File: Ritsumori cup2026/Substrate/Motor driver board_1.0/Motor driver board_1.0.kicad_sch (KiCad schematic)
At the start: 49 parts, among them J1 main, U1 DRV8412, U2 DRV8412

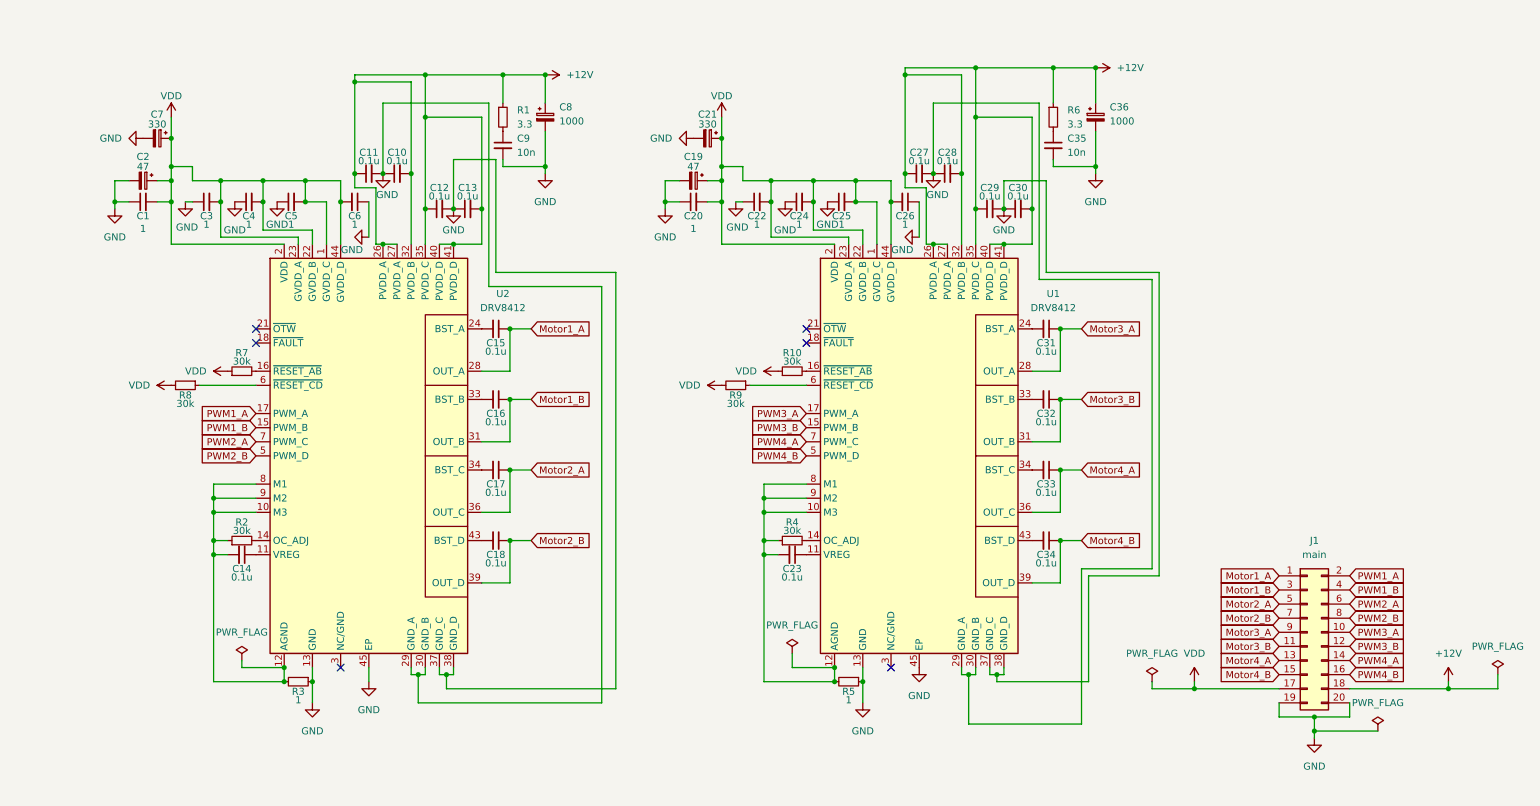
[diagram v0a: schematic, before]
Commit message: Auto Backup: 2026/03/24 15:00:23.58
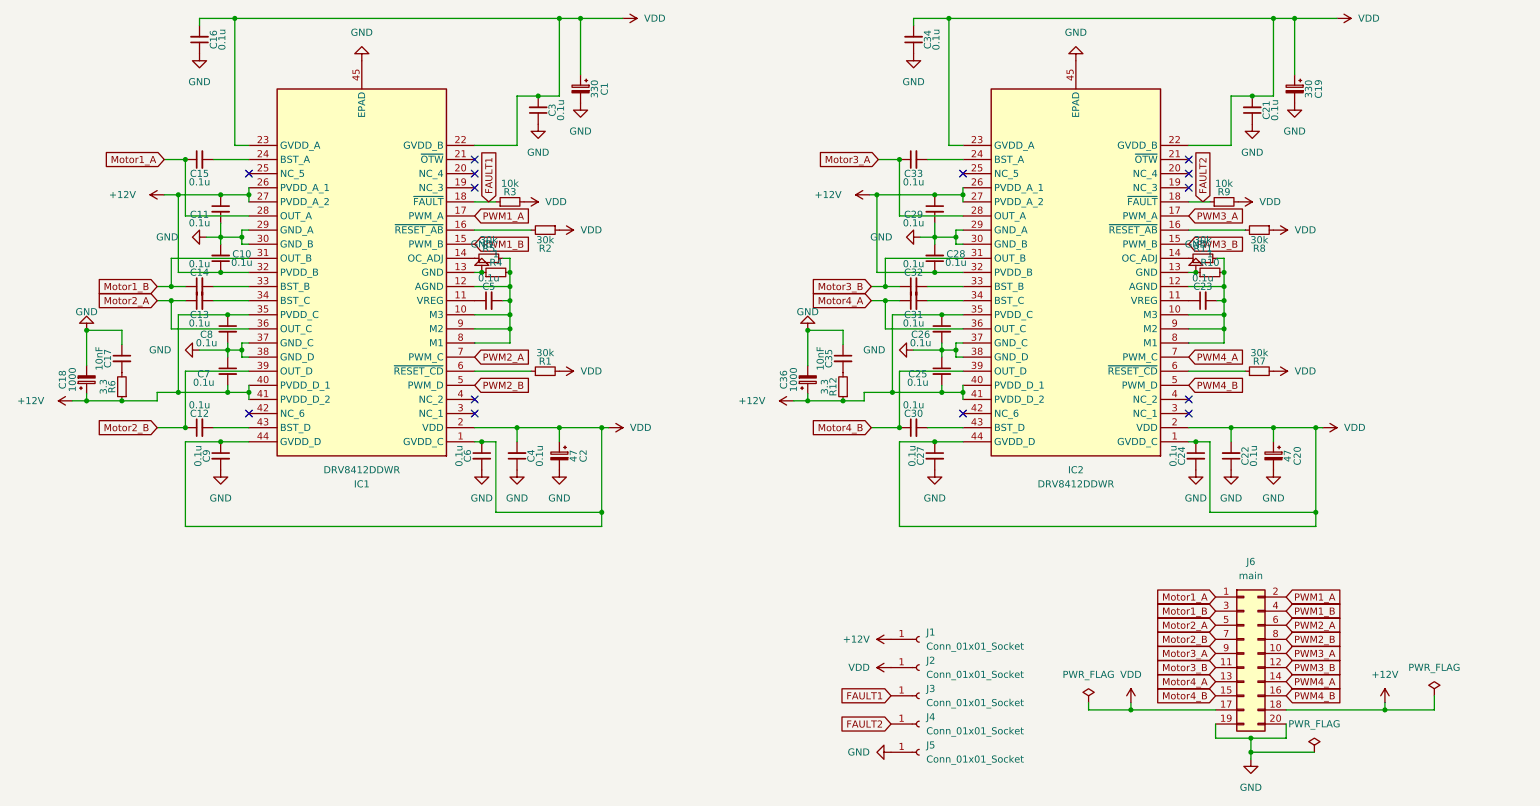
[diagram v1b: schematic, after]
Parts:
- removed C1, C20: 1, Capacitor_SMD:C_0603_1608Metric, symbol Device:C_Small
- removed C18: 0.1u, Capacitor_SMD:C_0603_1608Metric, symbol Device:C_Small
- removed C21, C7: 330, Capacitor_THT:CP_Radial_D10.0mm_P5.00mm, symbol Device:C_Polarized_Small
- removed C8: 1000, Capacitor_THT:CP_Radial_D10.0mm_P5.00mm, symbol Device:C_Polarized_Small
- removed U1, U2: DRV8412, Package_SO:HTSSOP-44-1EP_6.1x14mm_P0.635mm_EP5.2x14mm_Mask4.31x8.26mm_ThermalVias, symbol Driver_Motor:DRV8412
- added C1: 330, Capacitor_THT:CP_Radial_D10.0mm_P5.00mm, symbol Device:C_Polarized_Small
- added C18: 1000, Capacitor_THT:CP_Radial_D10.0mm_P5.00mm, symbol Device:C_Polarized_Small
- added C20: 47, Capacitor_THT:CP_Radial_D6.3mm_P2.50mm, symbol Device:C_Polarized_Small
- added C21, C7, C8: 0.1u, Capacitor_SMD:C_0603_1608Metric, symbol Device:C_Small
- added IC1, IC2: DRV8412DDWR, Package_SO:HTSSOP-44-1EP_6.1x14mm_P0.635mm_EP5.2x14mm_Mask4.31x8.26mm, symbol DRV8412DDWR:DRV8412DDWR
- added J1, J2, J3, J4, J5: Conn_01x01_Socket, TestPoint:TestPoint_Keystone_5000-5004_Miniature, symbol Connector:Conn_01x01_Socket
- added R11: 30k, Resistor_SMD:R_0603_1608Metric, symbol Device:R_Small
- added R12: 3.3, Resistor_SMD:R_0603_1608Metric, symbol Device:R_Small
- C17: value 0.1u -> 10nF
- C19: value 47 -> 330; footprint Capacitor_THT:CP_Radial_D6.3mm_P2.50mm -> Capacitor_THT:CP_Radial_D10.0mm_P5.00mm
- C22, C24, C25, C26, C3, C4, C5, C6: value 1 -> 0.1u
- C35: value 10n -> 10nF
- C9: value 10n -> 0.1u
- R1: value 3.3 -> 30k
- R10, R4: value 30k -> 1
- R3: value 1 -> 10k
- R5: value 1 -> 30k
- R9: value 30k -> 10k
- renumbered J1 to J6
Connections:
- net +12V: now also C10.1, C25.2, C26.1, C28.1, C18.1, C7.2, C8.1, IC1.26 (PVDD_A_1), IC1.27 (PVDD_A_2), IC1.32 (PVDD_B), IC1.35 (PVDD_C), IC1.40 (PVDD_D_1), IC1.41 (PVDD_D_2), IC2.26 (PVDD_A_1), IC2.27 (PVDD_A_2), IC2.32 (PVDD_B), IC2.35 (PVDD_C), IC2.40 (PVDD_D_1), IC2.41 (PVDD_D_2), J1.1 (Pin_1), R12.1; no longer C10.2, C12.1, C13.2, C27.1, C28.2, C30.2, R1.1
- net GND: now also C10.2, C16.1, C17.1, C24.2, C26.2, C28.2, C34.1, C35.1, C6.2, R10.1, R4.1, C1.2, C18.2, C20.2, C21.1, C7.1, C8.2, IC1.13 (GND), IC1.29 (GND_A), IC1.30 (GND_B), IC1.37 (GND_C), IC1.38 (GND_D), IC1.45 (EPAD), IC2.13 (GND), IC2.29 (GND_A), IC2.30 (GND_B), IC2.37 (GND_C), IC2.38 (GND_D), IC2.45 (EPAD), J5.1 (Pin_1); no longer C10.1, C12.2, C13.1, C24.1, C26.1, C28.1, C30.1, C35.2, C5.1, C6.1, R3.1, R5.1
- net Motor1_A: now also IC1.28 (OUT_A)
- net Motor1_B: now also C14.1, IC1.31 (OUT_B); no longer C16.1
- net Motor2_A: now also C13.1, IC1.36 (OUT_C); no longer C17.1
- net Motor2_B: now also C12.1, IC1.39 (OUT_D)
- net Motor3_A: now also C33.1, IC2.28 (OUT_A); no longer C31.1
- net Motor3_B: now also IC2.31 (OUT_B)
- net Motor4_A: now also C31.1, IC2.36 (OUT_C); no longer C33.1
- net Motor4_B: now also C30.1, IC2.39 (OUT_D); no longer C34.1
- net PWM1_A: now also IC1.17 (PWM_A)
- net PWM1_B: now also IC1.15 (PWM_B)
- net PWM2_A: now also IC1.7 (PWM_C)
- net PWM2_B: now also IC1.5 (PWM_D)
- net PWM3_A: now also IC2.17 (PWM_A)
- net PWM3_B: now also IC2.15 (PWM_B)
- net PWM4_A: now also IC2.7 (PWM_C)
- net PWM4_B: now also IC2.5 (PWM_D)
- net VDD: now also C16.2, C24.1, C27.1, C34.2, C6.1, C9.1, R1.2, R2.1, R3.2, R7.2, R8.1, C1.1, C20.1, C21.2, IC1.1 (GVDD_C), IC1.2 (VDD), IC1.22 (GVDD_B), IC1.23 (GVDD_A), IC1.44 (GVDD_D), IC2.1 (GVDD_C), IC2.2 (VDD), IC2.22 (GVDD_B), IC2.23 (GVDD_A), IC2.44 (GVDD_D), J2.1 (Pin_1); no longer C24.2, C25.2, C26.2, C5.2, C6.2, R10.1, R7.1, R8.2
- net at R10.2: now also C23.2, IC2.10 (M3), IC2.12 (AGND), IC2.8 (M1), IC2.9 (M2), R11.1
- net at C33.2: now also IC2.24 (BST_A)
- net at C15.2: now also IC1.24 (BST_A)
- net at C23.1: now also IC2.11 (VREG)
- net FAULT2: now reaches R9.1
- net FAULT2: now also IC2.18 (~{FAULT}), J4.1 (Pin_1)
- net at R2.2: now also IC1.16 (~{RESET_AB})
- net at C17.2: now also R6.2
- net at R4.2: now also C5.2, R5.2, IC1.10 (M3), IC1.12 (AGND), IC1.8 (M1), IC1.9 (M2)
- net at C31.2: now also IC2.34 (BST_C)
- net at C32.2: now also IC2.33 (BST_B)
- new net: C12.2, IC1.43 (BST_D)
- new net: C5.1, IC1.11 (VREG)
- new net: IC1.14 (OC_ADJ), R5.1
- new net: C14.2, IC1.33 (BST_B)
- new net: C13.2, IC1.34 (BST_C)
- new net: IC1.6 (~{RESET_CD}), R1.1
- new net: IC2.16 (~{RESET_AB}), R8.2
- new net: C35.2, R12.2
- new net: IC2.14 (OC_ADJ), R11.2
- new net: IC2.6 (~{RESET_CD}), R7.1
- new net: C30.2, IC2.43 (BST_D)
- new net FAULT1: IC1.18 (~{FAULT}), J3.1 (Pin_1), R3.1
- no-connect marks 6 -> 14
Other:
- moved on the sheet: J6
